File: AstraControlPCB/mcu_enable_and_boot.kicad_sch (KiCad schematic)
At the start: 13 parts, among them SW1 TS_Basic_Small, SW2 TS_Basic_Small

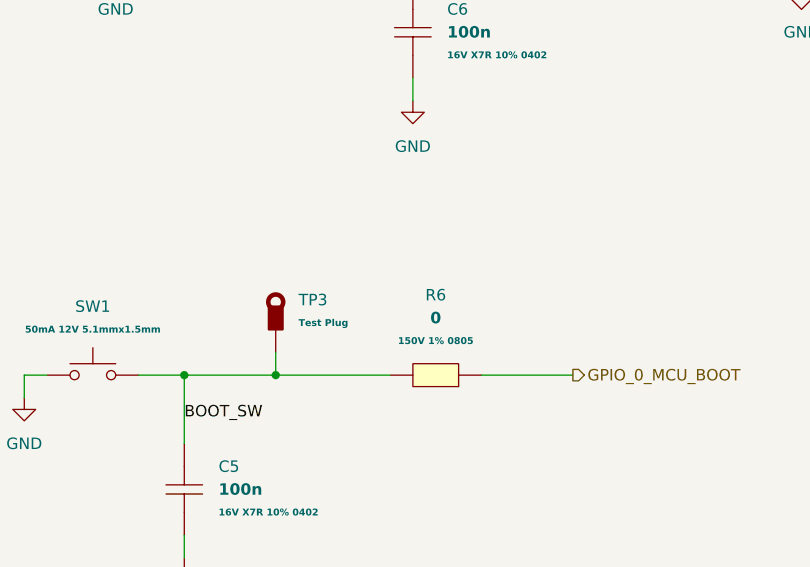
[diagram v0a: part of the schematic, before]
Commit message: Finished cleanup
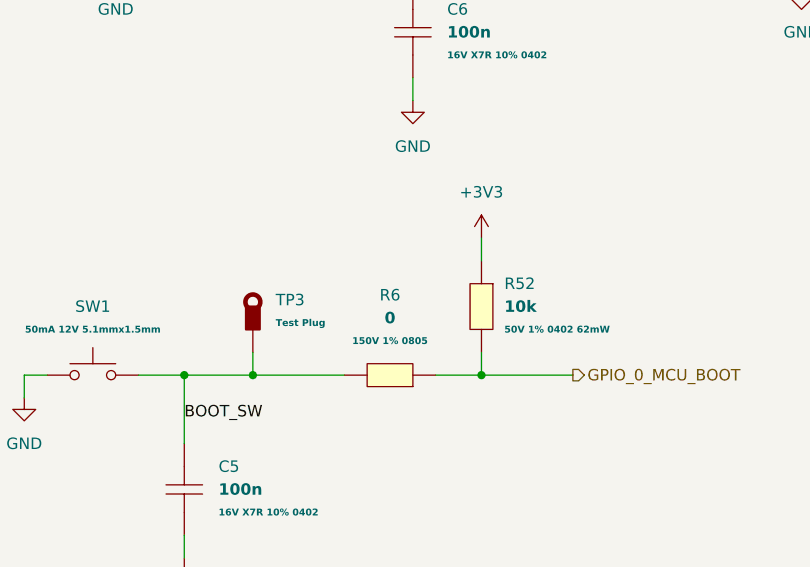
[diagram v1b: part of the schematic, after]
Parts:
- added R52: 10k, LiveAstra:R_0402_1005Metric, symbol LiveAstra:R_10kOhm_0402_62mW
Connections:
- net +3V3: now also R52.1
- net GPIO_0_MCU_BOOT: now also R52.2
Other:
- moved on the sheet: R6, TP3
